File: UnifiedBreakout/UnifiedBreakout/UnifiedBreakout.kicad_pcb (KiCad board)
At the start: 2 copper layers, 172.7 x 127.1 mm, 49 parts, among them J1 Dual DA15 Stacked, J2 ARGON J5, J4 PENDANT, J5 24V BUS, J6 DRAWBAR+MIST+AXIS_PWR, J7 LIMIT, J8 DB25_Receptacle_Dual, J9 AUX, U11 ILD74, U12 ILD74, U13 ILD74, U6 G3VM-61A1, U7 G3VM-61A1, U8 G3VM-61A1, U9 4N35

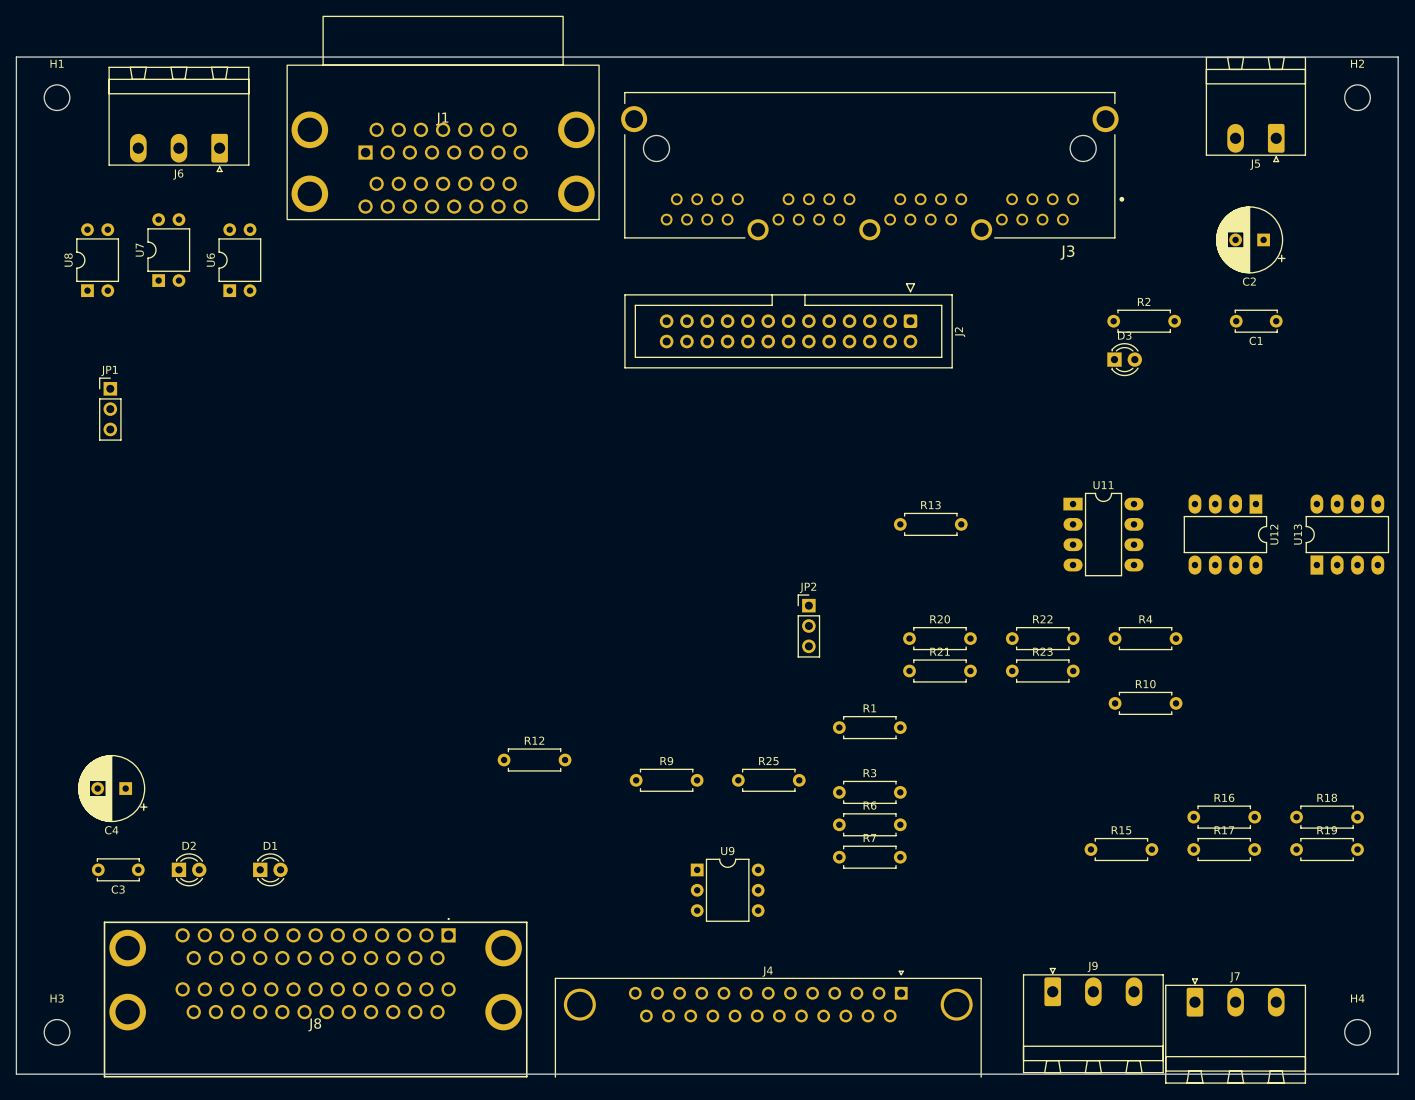
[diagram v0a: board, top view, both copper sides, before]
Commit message: Started some layout
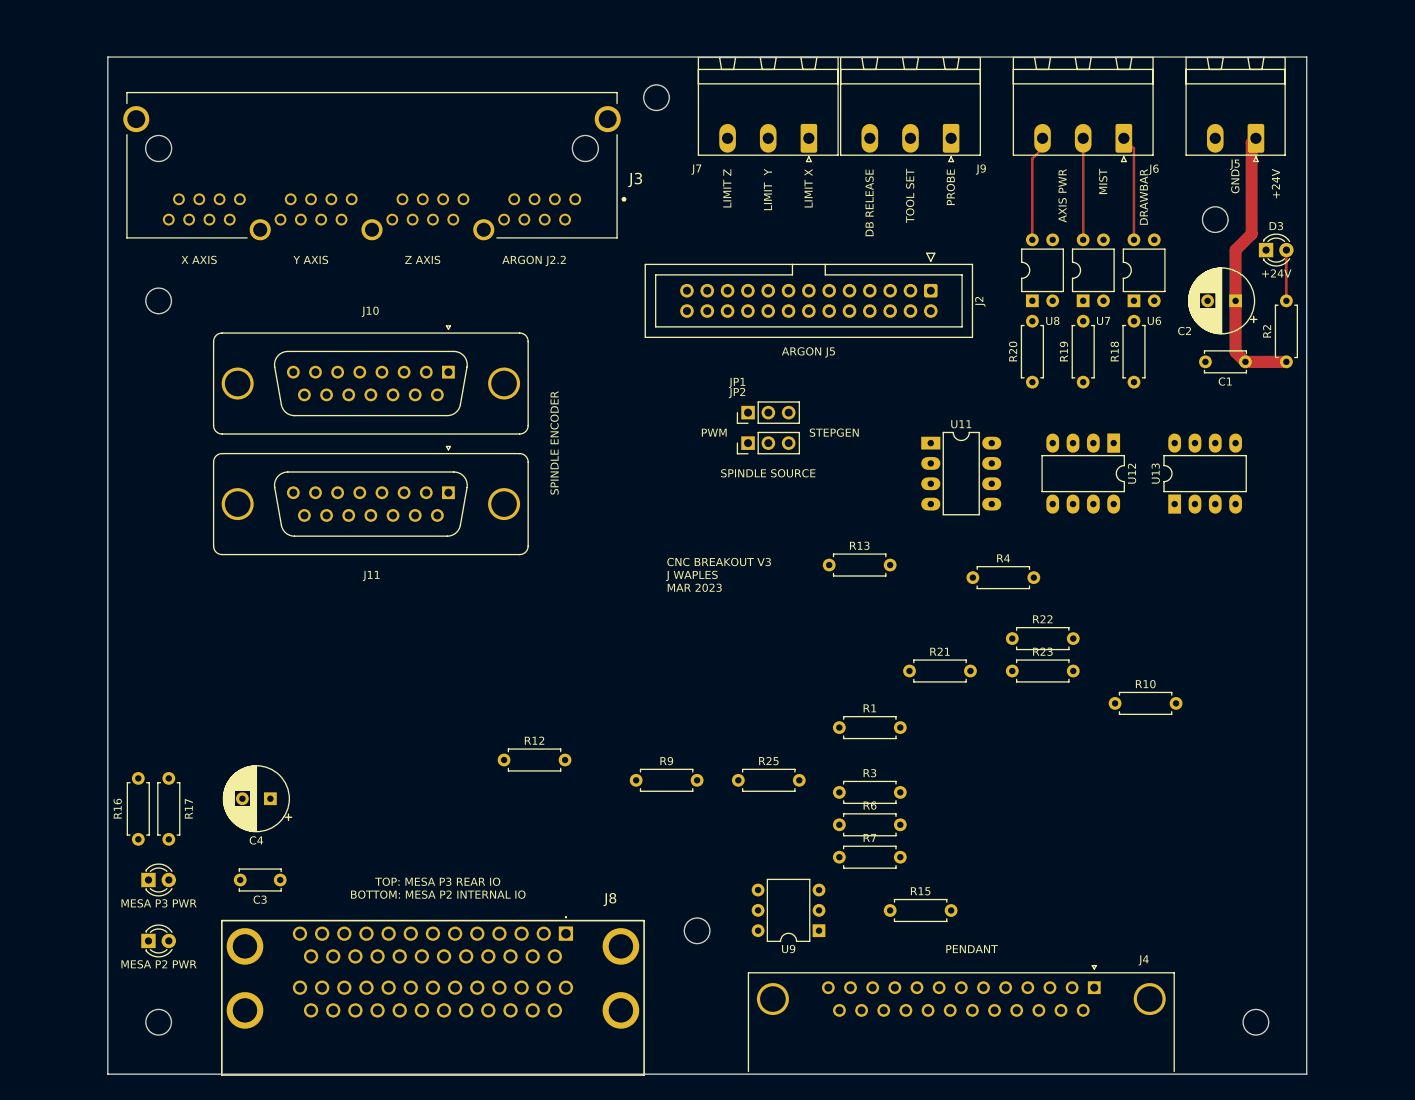
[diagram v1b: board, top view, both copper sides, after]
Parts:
- removed J1: Dual DA15 Stacked, UnifiedBreakout:NorComp-Dual-DA15
- added H5: MountingHole, MountingHole:MountingHole_3.2mm_M3, F.Cu at (97.8, 43.2)
- added H6: MountingHole, MountingHole:MountingHole_3.2mm_M3, F.Cu at (172.7, 158.8)
- added J10: DA15_Receptacle_MountingHoles, Connector_Dsub:DSUB-15_Female_Vertical_P2.77x2.84mm_MountingHoles, F.Cu at (71.8, 77.5)
- added J11: DA15_Receptacle_MountingHoles, Connector_Dsub:DSUB-15_Female_Vertical_P2.77x2.84mm_MountingHoles, F.Cu at (71.8, 92.6)
- moved R17 132.2 mm to (33.0, 128.3), turned to -90 degrees
- moved R16 128.2 mm to (36.8, 135.9), turned to 90 degrees
- moved J7 118.3 mm to (116.8, 48.3), turned to 180 degrees
- moved U8 118.1 mm to (144.8, 68.6)
- moved U7 115.6 mm to (151.1, 68.6)
- moved U6 113.0 mm to (157.5, 68.6)
- moved J6 113.0 mm to (156.2, 48.3)
- moved J9 107.4 mm to (134.6, 48.3), turned to 180 degrees
- moved H4 83.5 mm to (102.9, 147.3)
- moved JP1 79.8 mm to (109.2, 82.5), turned to 90 degrees
- moved R19 64.2 mm to (151.1, 78.7), turned to 90 degrees
- moved J3 62.2 mm to (62.2, 49.5)
- moved R18 58.0 mm to (157.5, 78.7), turned to 90 degrees
- moved R20 35.5 mm to (144.8, 78.7), turned to 90 degrees
- moved H1 28.4 mm to (35.6, 68.6)
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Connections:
- J3 pad 1_1: GND -> +24V
- J3 pad 1_4: +24V -> GND
- J3 pad 2_1: /MESA P3 REAR IO/IO_02_STEPGEN_00_STEP -> unconnected-(J3A-P2_1-Pad2_1)
- J3 pad 2_2: /MESA P3 REAR IO/IO_06_STEPGEN_01_STEP -> /MESA P3 REAR IO/IO_09_STEPGEN_02_STEP
- J3 pad 2_3: /MESA P3 REAR IO/IO_09_STEPGEN_02_STEP -> /MESA P3 REAR IO/IO_06_STEPGEN_01_STEP
- J3 pad 2_4: unconnected-(J3D-P2_4-Pad2_4) -> /MESA P3 REAR IO/IO_02_STEPGEN_00_STEP
- J3 pad 3_1: GND -> /ARGON ESTOP/RS485_A
- J3 pad 3_4: /ARGON ESTOP/RS485_A -> GND
- J3 pad 4_1: /MESA P3 REAR IO/IO_04_STEPGEN_00_DIR -> /ARGON ESTOP/ESTOP+
- J3 pad 4_2: /MESA P3 REAR IO/IO_08_STEPGEN_01_DIR -> /MESA P3 REAR IO/IO_10_STEPGEN_02_DIR
- J3 pad 4_3: /MESA P3 REAR IO/IO_10_STEPGEN_02_DIR -> /MESA P3 REAR IO/IO_08_STEPGEN_01_DIR
- J3 pad 4_4: /ARGON ESTOP/ESTOP+ -> /MESA P3 REAR IO/IO_04_STEPGEN_00_DIR
- J3 pad 6_1: /X MOT/ENABLE -> /ARGON ESTOP/RS485_B
- J3 pad 6_2: /Y MOT/ENABLE -> /Z MOT/ENABLE
- J3 pad 6_3: /Z MOT/ENABLE -> /Y MOT/ENABLE
- J3 pad 6_4: /ARGON ESTOP/RS485_B -> /X MOT/ENABLE
- J3 pad 7_1: GND -> +24V
- J3 pad 7_4: +24V -> GND
- J3 pad 8_1: /ALARM -> GND
- J3 pad 8_4: GND -> /ALARM
- J3 pad S1: GND -> Net-(J3A-SHIELD-PadS1)
- J3 pad S2: GND -> Net-(J3A-SHIELD-PadS1)
- J3 pad S3: GND -> Net-(J3A-SHIELD-PadS1)
- J3 pad S4: GND -> Net-(J3A-SHIELD-PadS1)
- J3 pad S5: GND -> Net-(J3A-SHIELD-PadS1)
- J8 pad MH4: unconnected-(J8-PadMH4) -> GND
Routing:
- net +24V: track 0.00 -> 34.6 mm
- net Net-(J6-Pin_3): track 0.00 -> 13.2 mm
- net Net-(J6-Pin_1): track 0.00 -> 13.2 mm
- net Net-(J6-Pin_2): track 0.00 -> 12.7 mm
- net Net-(D3-A): track 0.00 -> 6.35 mm
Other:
- board size 172.7 x 127.1 mm -> 149.9 x 127.1 mm
- board text added: "+24V"
- board text added: "ARGON J2.2"
- board text added: "ARGON J5"
- board text added: "AXIS PWR"
- board text added: "CNC BREAKOUT V3 J WAPLES MAR 2023"
- board text added: "DB RELEASE"
- board text added: "DRAWBAR"
- board text added: "GND"
- board text added: "LIMIT X"
- board text added: "LIMIT Y"
- board text added: "LIMIT Z"
- board text added: "MIST"
- board text added: "PENDANT"
- board text added: "PROBE"
- board text added: "PWM"
- board text added: "SPINDLE ENCODER"
- board text added: "SPINDLE SOURCE"
- board text added: "STEPGEN"
- board text added: "TOOL SET"
- board text added: "TOP: MESA P3 REAR IO BOTTOM: MESA P2 INTERNAL IO"
- board text added: "X AXIS"
- board text added: "Y AXIS"
- board text added: "Z AXIS"
